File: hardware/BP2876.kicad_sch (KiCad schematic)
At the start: 12 parts, among them U301 BP2876

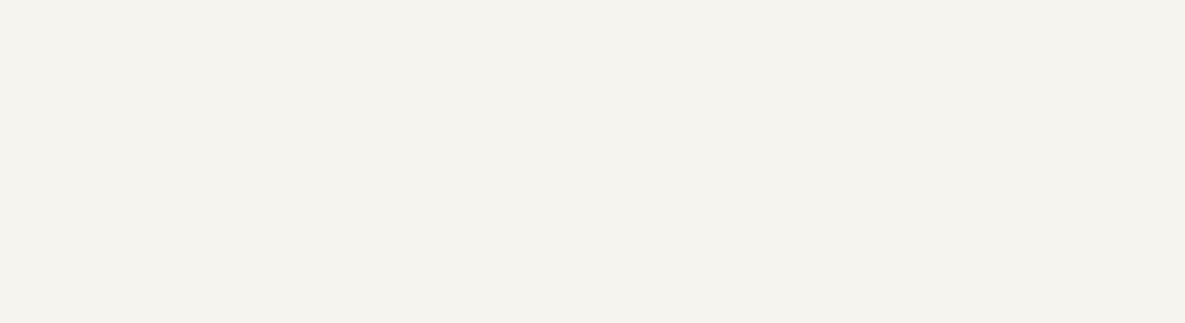
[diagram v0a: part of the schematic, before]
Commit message: BP2956XS
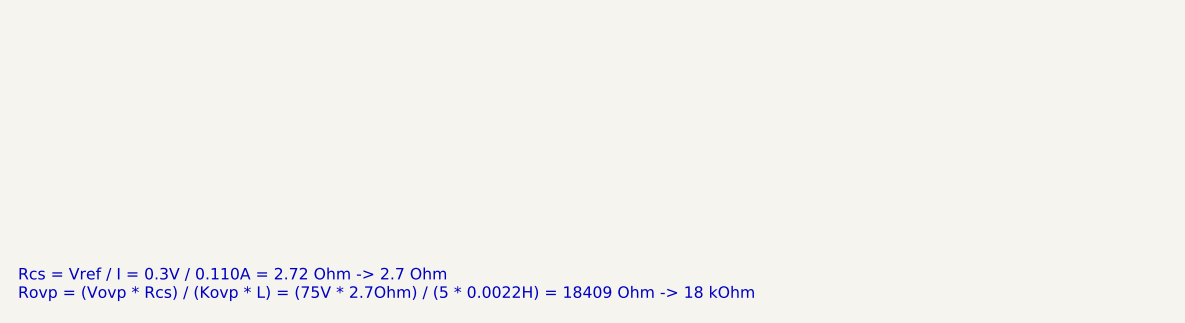
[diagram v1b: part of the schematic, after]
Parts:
- U301: Datasheet CN https://taoic.oss-cn-hangzhou.aliyuncs.com/9208/product/HZD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 -> (none)
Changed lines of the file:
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@@
 	(generator_version "9.0")
 	(paper "A4")
+	(text_box "Rcs = Vref / I = 0.3V / 0.110A = 2.72 Ohm -> 2.7 Ohm\nRovp = (Vovp * Rcs) / (Kovp * L) = (75V * 2.7Ohm) / (5 * 0.0022H) = 18409 Ohm -> 18 kOhm"
+		(exclude_from_sim no)
+		(at 50.8 177.8 0)
+		(size 111.76 6.35)
+		(margins 0.9525 0.9525 0.9525 0.9525)
+		(stroke
+			(width -0.0001)
+			(type solid)
+		)
+		(fill
+			(type none)
+		)
+		(effects
+			(font
+				(size 1.27 1.27)
+			)
+			(justify left top)
+		)
+	)
 	(junction
 		(at 238.76 69.85)
@@
 			)
 		)
-		(property "Datasheet" "kicad-embed://BP2876D.PDF"
+		(property "Datasheet" "https://taoic.oss-cn-hangzhou.aliyuncs.com/9208/product/HZDZ88_1636526643000.pdf"
 			(at 198.882 74.168 0)
 			(effects
@@
 			(effects
 				(font
-					(size 1.27 1.27)
-				)
-				(hide yes)
-			)
-		)
-		(property "Datasheet CN" "https://taoic.oss-cn-hangzhou.aliyuncs.com/9208/product/HZDZ88_1636526643000.pdf"
-			(at 199.898 103.124 0)
-			(effects
-				(font
